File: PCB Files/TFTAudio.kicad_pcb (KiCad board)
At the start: 2 copper layers, 118 x 53.5 mm, 57 parts, among them J1 USB_C_Receptacle_USB2.0_14P, J2 Conn_01x02, J3 Conn_01x14_Socket, J5 Conn_01x12_Pin, Q1 BSS138, Q2 BSS138, Q3 DMG2301L, SW1 SW_SPST, U1 ESP32-WROVER-E, U2 CH340C, U3 MCP73831-2-OT, U4 AP2112K-3.3, U5 PCM5102A, X1 STEREO_AUDIO_JACK

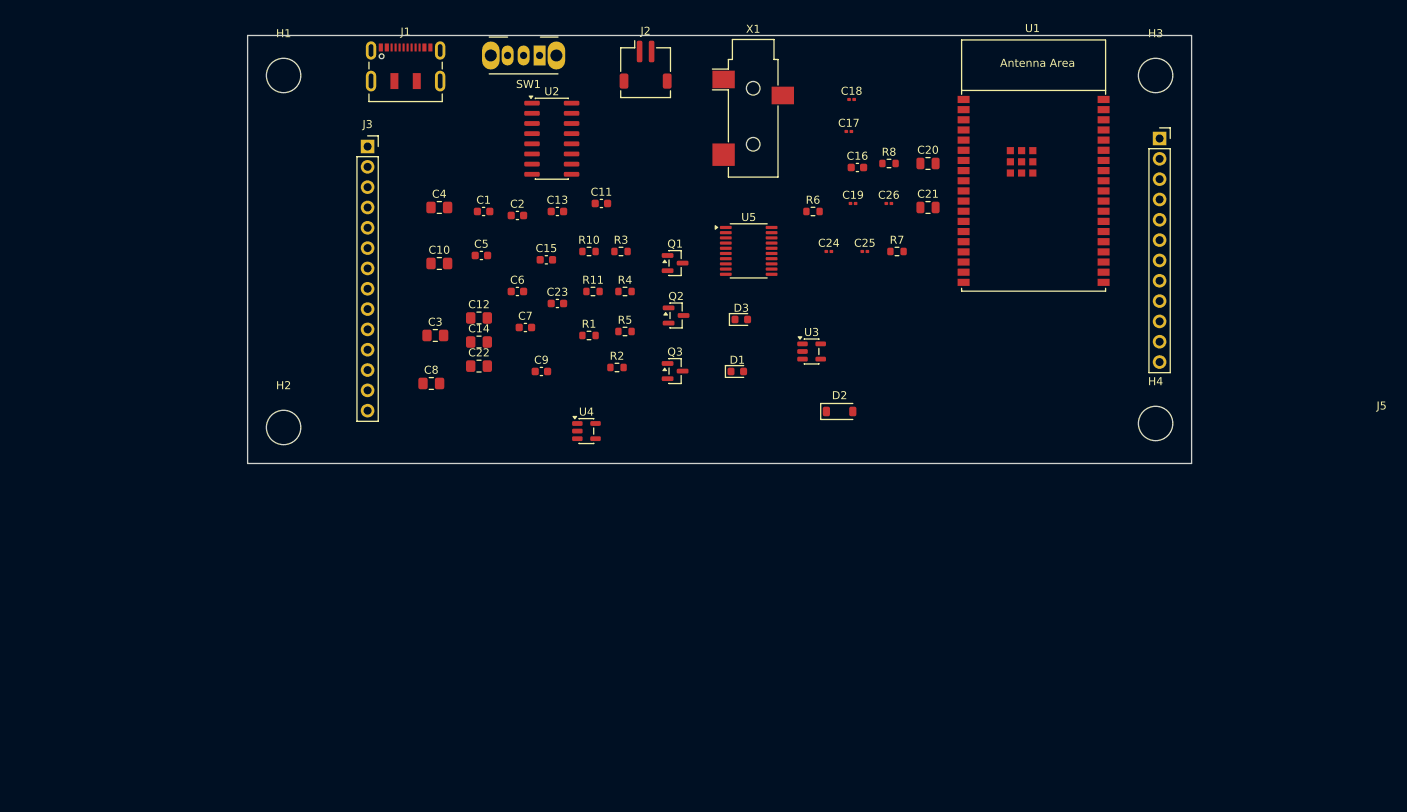
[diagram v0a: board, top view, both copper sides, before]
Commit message: Mark R Commit - PCB help
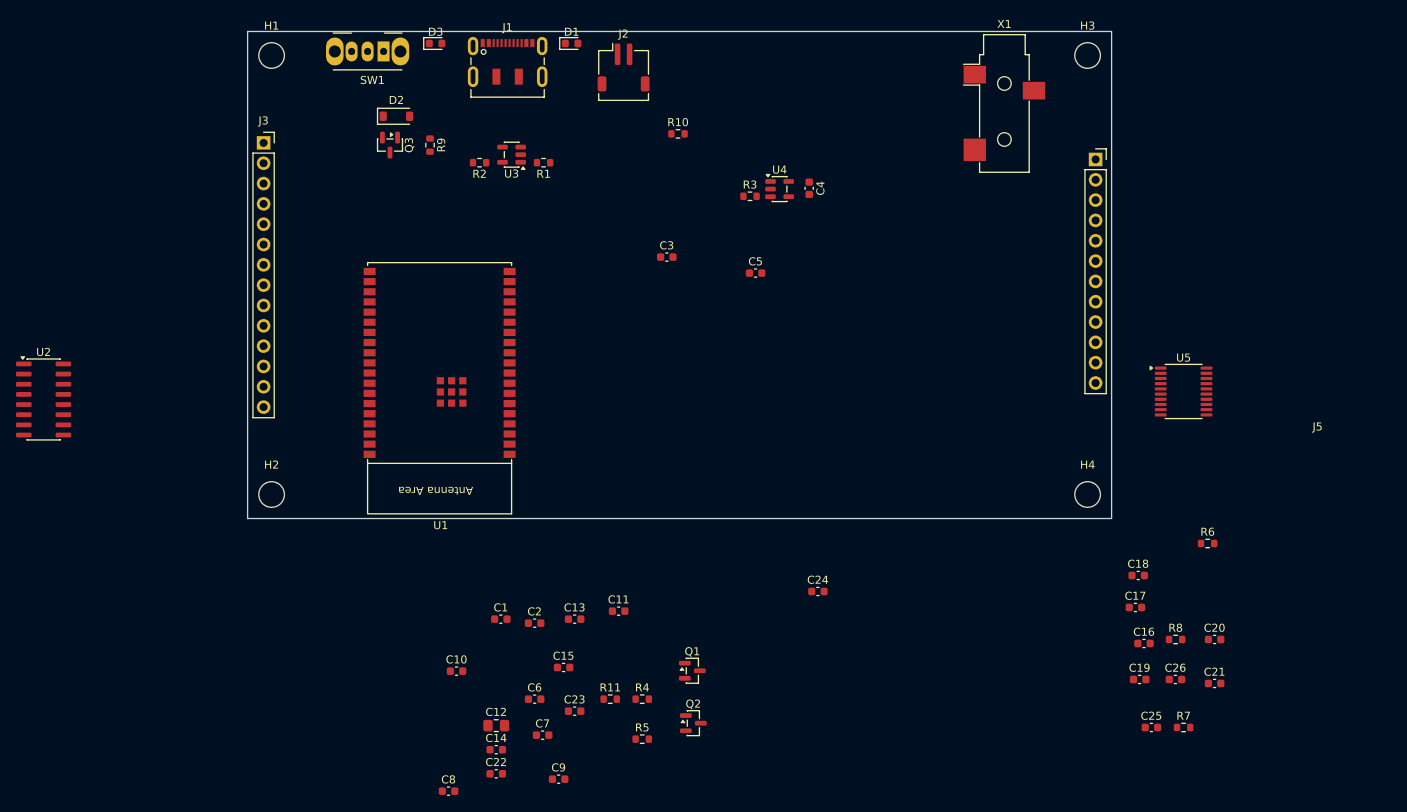
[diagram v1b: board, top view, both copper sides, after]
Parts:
- added R9: 100k, Resistor_SMD:R_0603_1608Metric, F.Cu at (35.8, 32.2)
- C10, C14, C22, C3, C4, C8: footprint Capacitor_SMD:C_0805_2012Metric_Pad1.18x1.45mm_HandSolder -> Capacitor_SMD:C_0603_1608Metric
- C17, C18, C19, C24, C25, C26: footprint Capacitor_SMD:C_0201_0603Metric -> Capacitor_SMD:C_0603_1608Metric
- C20, C21: footprint Capacitor_SMD:C_0805_2012Metric -> Capacitor_SMD:C_0603_1608Metric
- D1: value LED -> Charge
- H1, H2, H3, H4: footprint MountingHole:MountingHole_4.3mm_M4 -> MountingHole:MountingHole_3.2mm_M3_ISO14580
- J2: value Conn_01x02 -> Lipo 1S
- J3: value Conn_01x14_Socket -> Display
- J5: value Conn_01x12_Pin -> expansion
- moved U1 79.3 mm to (37.0, 62.6), turned to 180 degrees
- moved U2 71.4 mm to (-12.5, 64.0)
- moved C16 69.5 mm to (125.0, 94.5)
- moved C17 69.5 mm to (124.0, 90.0)
- moved C18 69.5 mm to (124.3, 86.0)
- moved C20 69.5 mm to (133.9, 94.0)
- moved C21 69.5 mm to (133.9, 99.5)
- moved C25 69.5 mm to (126.0, 105.0)
- moved R7 69.5 mm to (130.0, 105.0)
- moved R8 69.5 mm to (129.0, 94.0)
- moved C19 69.5 mm to (124.5, 99.0)
- moved C26 69.5 mm to (129.0, 99.0)
- moved D2 66.6 mm to (31.6, 28.6)
- moved R6 64.5 mm to (133.0, 82.0)
- moved U5 57.1 mm to (130.0, 63.0)
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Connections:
- net Net-(D2-K) renamed /SWIN
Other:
- board size 118 x 53.5 mm -> 108 x 60.9 mm
